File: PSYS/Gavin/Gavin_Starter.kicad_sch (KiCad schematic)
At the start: 24 parts, among them J1 Conn_Coaxial, J2 Conn_ARM_SWD_TagConnect_TC2030, U1 STM32WB55CEUx, X1 32MHz, X2 32Khz768

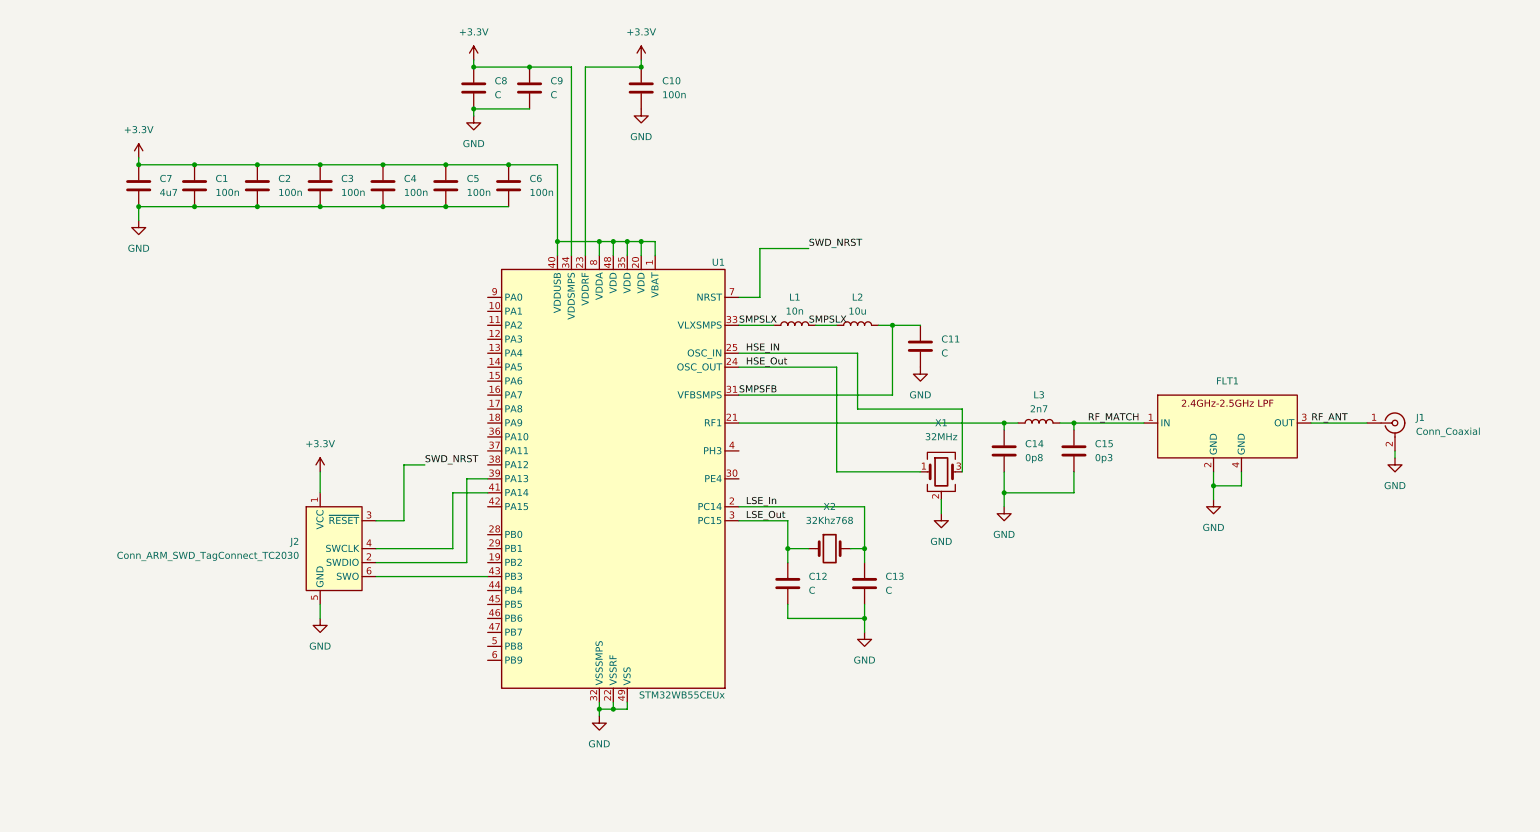
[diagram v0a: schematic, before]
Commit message: schematic1
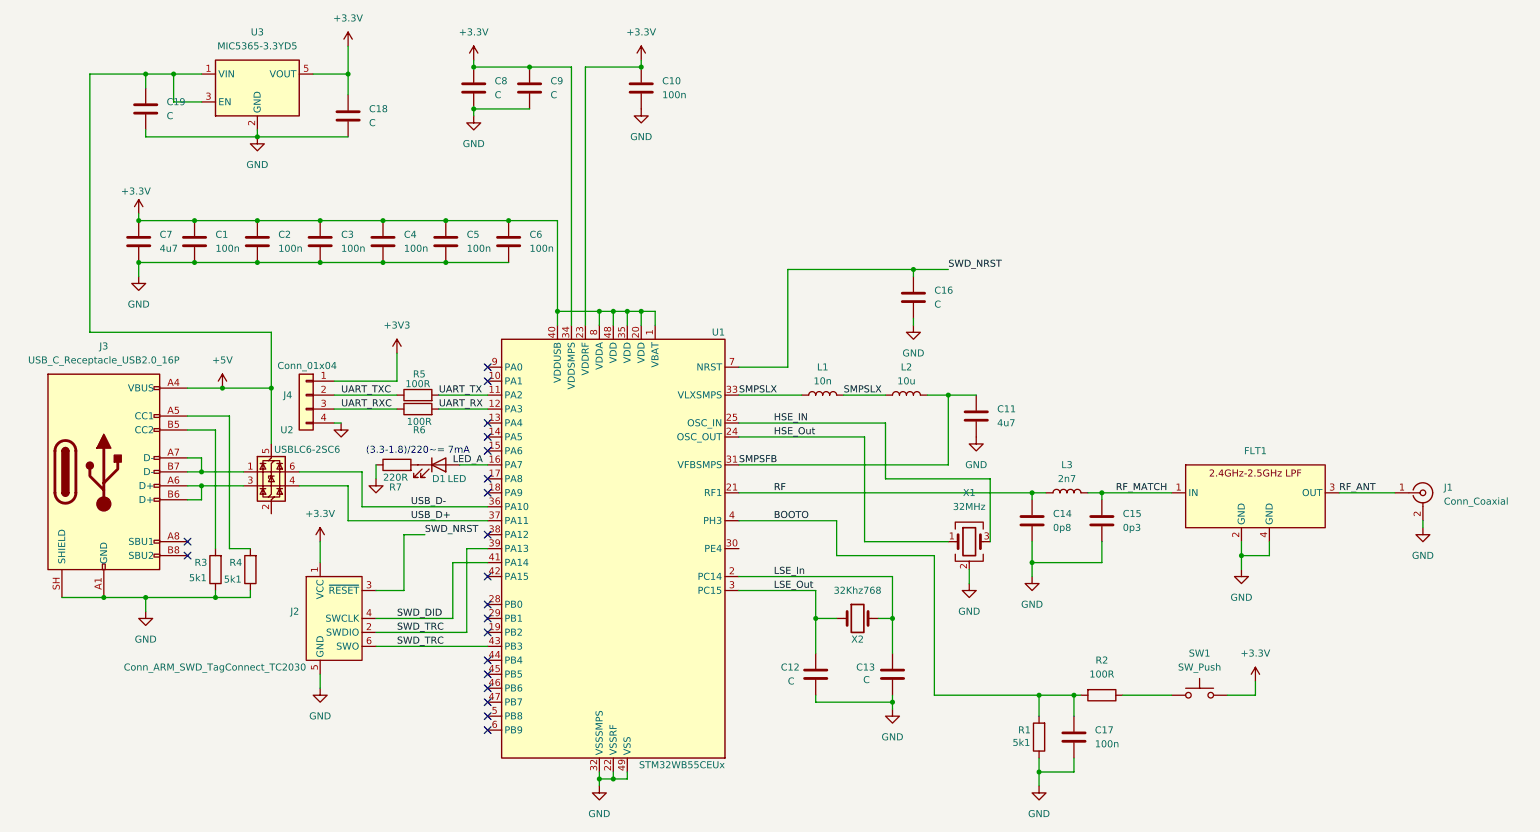
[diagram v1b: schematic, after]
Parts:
- added C16, C18, C19: C, symbol Device:C
- added C17: 100n, symbol Device:C
- added D1: LED, symbol Device:LED
- added J3: USB_C_Receptacle_USB2.0_16P, symbol Connector:USB_C_Receptacle_USB2.0_16P
- added J4: Conn_01x04, symbol Connector_Generic:Conn_01x04
- added R1, R3, R4: 5k1, symbol Device:R
- added R2, R5, R6: 100R, symbol Device:R
- added R7: 220R, symbol Device:R
- added SW1: SW_Push, symbol Switch:SW_Push
- added U2: USBLC6-2SC6, Package_TO_SOT_SMD:SOT-23-6, symbol Power_Protection:USBLC6-2SC6
- added U3: MIC5365-3.3YD5, Package_TO_SOT_SMD:TSOT-23-5, symbol Regulator_Linear:MIC5365-3.3YD5
- C11: value C -> 4u7
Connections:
- net +3.3V: now also C18.1, SW1.2, U3.5 (VOUT)
- net GND: now also C16.2, C17.2, C18.2, C19.2, J3.A1 (GND), J3.A12 (GND), J3.B1 (GND), J3.B12 (GND), J3.SH (SHIELD), J4.4 (Pin_4), R1.1, R3.1, R4.1, R7.1, U3.2 (GND)
- net SMPSLX: now also L1.2, L2.1
- net SWD_NRST: now also C16.1
- net RF: now reaches C14.1, L3.1, U1.21 (RF1)
- net UART_TX: now reaches U1.11 (PA2)
- net UART_TX: now also R5.2
- net UART_RX: now reaches U1.12 (PA3)
- net UART_RX: now also R6.2
- net at U1.16 (PA7): now also D1.2 (A)
- net USB_D-: now reaches U1.36 (PA10)
- net USB_D-: now also U2.6 (I/O1)
- net USB_D+: now reaches U1.37 (PA11)
- net USB_D+: now also U2.4 (I/O2)
- net SWD_TRC: now reaches J2.2 (SWDIO), U1.39 (PA13)
- net SWD_TRC: now also J2.6 (SWO), U1.43 (PB3)
- net BOOTO: now reaches U1.4 (PH3)
- net BOOTO: now also C17.1, R1.2, R2.2
- net SWD_DID: now reaches J2.4 (SWCLK), U1.41 (PA14)
- new net: J3.B5 (CC2), R3.2
- new net: J3.A5 (CC1), R4.2
- new net: J3.A6 (D+), J3.B6 (D+), U2.3 (I/O2)
- new net: J3.A7 (D-), J3.B7 (D-), U2.1 (I/O1)
- new net: R2.1, SW1.1
- new net: D1.1 (K), R7.2
- new net +3V3: J4.1 (Pin_1)
- new net +5V: C19.1, J3.A4 (VBUS), J3.A9 (VBUS), J3.B4 (VBUS), J3.B9 (VBUS), U2.5 (VBUS), U3.1 (VIN), U3.3 (EN)
- new net UART_RXC: J4.3 (Pin_3), R6.1
- new net UART_TXC: J4.2 (Pin_2), R5.1
- no-connect marks 0 -> 20
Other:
- note added: "(3.3-1.8)/220~= 7mA"
- moved on the sheet: C1, C11, C12, C13, C14, C15, C2, C3, C4, C5, C6, C7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
